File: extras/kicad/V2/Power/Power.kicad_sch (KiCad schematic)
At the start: 73 parts, among them J1 Conn_01x02, J2 Screw_Terminal_01x06, J3 Screw_Terminal_01x06, J4 Screw_Terminal_01x06, J5 Screw_Terminal_01x06, J6 Conn_02x20_Odd_Even, J7 Conn_02x20_Odd_Even, U1 TB6612FNG, U2 TB6612FNG, U3 TPS5430DDAR, U4 TPS5430DDAR

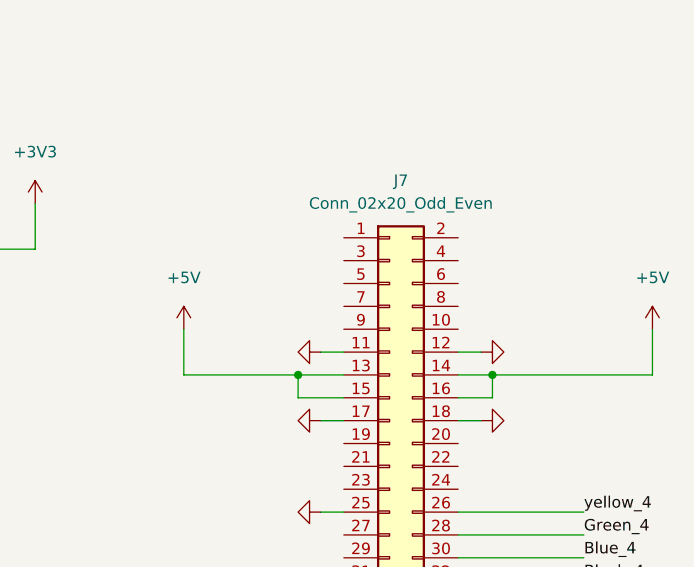
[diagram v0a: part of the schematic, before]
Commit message: g
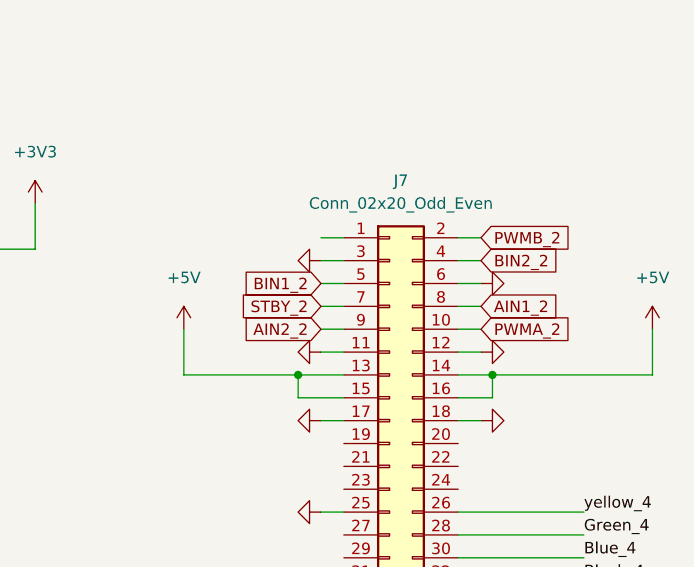
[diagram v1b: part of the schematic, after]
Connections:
- net AIN1_2: now also J7.8 (Pin_8)
- net AIN2_2: now also J7.9 (Pin_9)
- net BIN1_2: now also J7.5 (Pin_5)
- net BIN2_2: now also J7.4 (Pin_4)
- net GND: now also J7.3 (Pin_3), J7.6 (Pin_6)
- net PWMA_2: now also J7.10 (Pin_10)
- net PWMB_2: now also J7.2 (Pin_2)
- net STBY_2: now also J7.7 (Pin_7)
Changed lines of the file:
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@@
     (stroke (width 0) (type default) (color 0 0 0 0))
   )
+  (wire (pts (xy 363.22 119.38) (xy 365.76 119.38))
+    (stroke (width 0) (type default) (color 0 0 0 0))
+  )
+  (wire (pts (xy 363.22 124.46) (xy 365.76 124.46))
+    (stroke (width 0) (type default) (color 0 0 0 0))
+  )
   (wire (pts (xy 34.29 163.83) (xy 38.1 163.83))
     (stroke (width 0) (type default) (color 0 0 0 0))
@@
     (stroke (width 0) (type default) (color 0 0 0 0))
   )
+  (wire (pts (xy 378.46 124.46) (xy 381 124.46))
+    (stroke (width 0) (type default) (color 0 0 0 0))
+  )
   (wire (pts (xy 173.99 163.83) (xy 173.99 166.37))
     (stroke (width 0) (type default) (color 0 0 0 0))
@@
     (stroke (width 0) (type default) (color 0 0 0 0))
   )
+  (wire (pts (xy 378.46 129.54) (xy 381 129.54))
+    (stroke (width 0) (type default) (color 0 0 0 0))
+  )
   (wire (pts (xy 44.45 212.09) (xy 86.36 212.09))
     (stroke (width 0) (type default) (color 0 0 0 0))
@@
     (stroke (width 0) (type default) (color 0 0 0 0))
   )
+  (wire (pts (xy 363.22 127) (xy 365.76 127))
+    (stroke (width 0) (type default) (color 0 0 0 0))
+  )
   (wire (pts (xy 133.35 175.26) (xy 133.35 176.53))
     (stroke (width 0) (type default) (color 0 0 0 0))
@@
     (stroke (width 0) (type default) (color 0 0 0 0))
   )
+  (wire (pts (xy 363.22 121.92) (xy 365.76 121.92))
+    (stroke (width 0) (type default) (color 0 0 0 0))
+  )
   (wire (pts (xy 43.18 46.99) (xy 46.99 46.99))
     (stroke (width 0) (type default) (color 0 0 0 0))
@@
     (stroke (width 0) (type default) (color 0 0 0 0))
   )
+  (wire (pts (xy 378.46 119.38) (xy 381 119.38))
+    (stroke (width 0) (type default) (color 0 0 0 0))
+  )
+  (wire (pts (xy 378.46 127) (xy 381 127))
+    (stroke (width 0) (type default) (color 0 0 0 0))
+  )
   (wire (pts (xy 303.53 123.19) (xy 303.53 120.65))
     (stroke (width 0) (type default) (color 0 0 0 0))
@@
     (stroke (width 0) (type default) (color 0 0 0 0))
   )
+  (wire (pts (xy 363.22 129.54) (xy 365.76 129.54))
+    (stroke (width 0) (type default) (color 0 0 0 0))
+  )
   (wire (pts (xy 361.95 74.93) (xy 370.84 74.93))
     (stroke (width 0) (type default) (color 0 0 0 0))
@@
     (stroke (width 0) (type default) (color 0 0 0 0))
   )
+  (wire (pts (xy 378.46 121.92) (xy 381 121.92))
+    (stroke (width 0) (type default) (color 0 0 0 0))
+  )
   (wire (pts (xy 127 83.82) (xy 118.11 83.82))
     (stroke (width 0) (type default) (color 0 0 0 0))
@@
     )
   )
+  (global_label "PWMA_2" (shape input) (at 381 129.54 0) (fields_autoplaced)
+    (effects (font (size 1.27 1.27)) (justify left))
+    (property "Intersheet References" "${INTERSHEET_REFS}" (id 0) (at 390.8517 129.4606 0)
+      (effects (font (size 1.27 1.27)) (justify left) hide)
+    )
+  )
   (global_label "AIN2_2" (shape input) (at 171.45 93.98 180) (fields_autoplaced)
     (effects (font (size 1.27 1.27)) (justify right))
@@
     )
   )
+  (global_label "STBY_2" (shape input) (at 363.22 127 180) (fields_autoplaced)
+    (effects (font (size 1.27 1.27)) (justify right))
+    (property "Intersheet References" "${INTERSHEET_REFS}" (id 0) (at 354.094 126.9206 0)
+      (effects (font (size 1.27 1.27)) (justify right) hide)
+    )
+  )
   (global_label "BIN1_1" (shape input) (at 80.01 96.52 180) (fields_autoplaced)
     (effects (font (size 1.27 1.27)) (justify right))
@@
     )
   )
+  (global_label "AIN1_2" (shape input) (at 381 127 0) (fields_autoplaced)
+    (effects (font (size 1.27 1.27)) (justify left))
+    (property "Intersheet References" "${INTERSHEET_REFS}" (id 0) (at 389.8236 127.0794 0)
+      (effects (font (size 1.27 1.27)) (justify left) hide)
+    )
+  )
+  (global_label "BIN1_2" (shape input) (at 363.22 124.46 180) (fields_autoplaced)
+    (effects (font (size 1.27 1.27)) (justify right))
+    (property "Intersheet References" "${INTERSHEET_REFS}" (id 0) (at 354.215 124.3806 0)
+      (effects (font (size 1.27 1.27)) (justify right) hide)
+    )
+  )
   (global_label "STBY_2" (shape input) (at 172.72 78.74 180) (fields_autoplaced)
     (effects (font (size 1.27 1.27)) (justify right))
@@
     )
   )
+  (global_label "PWMB_2" (shape input) (at 381 119.38 0) (fields_autoplaced)
+    (effects (font (size 1.27 1.27)) (justify left))
+    (property "Intersheet References" "${INTERSHEET_REFS}" (id 0) (at 391.0331 119.4594 0)
+      (effects (font (size 1.27 1.27)) (justify left) hide)
+    )
+  )
   (global_label "BIN1_2" (shape input) (at 171.45 96.52 180) (fields_autoplaced)
     (effects (font (size 1.27 1.27)) (justify right))
@@
     )
   )
+  (global_label "BIN2_2" (shape input) (at 381 121.92 0) (fields_autoplaced)
+    (effects (font (size 1.27 1.27)) (justify left))
+    (property "Intersheet References" "${INTERSHEET_REFS}" (id 0) (at 390.005 121.9994 0)
+      (effects (font (size 1.27 1.27)) (justify left) hide)
+    )
+  )
   (global_label "AIN1_1" (shape input) (at 80.01 91.44 180) (fields_autoplaced)
     (effects (font (size 1.27 1.27)) (justify right))
@@
     )
   )
+  (global_label "AIN2_2" (shape input) (at 363.22 129.54 180) (fields_autoplaced)
+    (effects (font (size 1.27 1.27)) (justify right))
+    (property "Intersheet References" "${INTERSHEET_REFS}" (id 0) (at 354.3964 129.6194 0)
+      (effects (font (size 1.27 1.27)) (justify right) hide)
+    )
+  )
   (symbol (lib_id "power:GND") (at 110.49 116.84 0) (unit 1)
     (in_bom yes) (on_board yes) (fields_autoplaced)
@@
     (pin "1")
   )
+  (symbol (lib_id "power:GND") (at 381 124.46 90) (unit 1)
+    (in_bom yes) (on_board yes) (fields_autoplaced)
+    (property "Reference" "#PWR0129" (id 0) (at 387.35 124.46 0)
+      (effects (font (size 1.27 1.27)) hide)
+    )
+    (property "Value" "GND" (id 1) (at 385.445 124.46 0)
+      (effects (font (size 1.27 1.27)) hide)
+    )
+    (property "Footprint" "" (id 2) (at 381 124.46 0)
+      (effects (font (size 1.27 1.27)) hide)
+    )
+    (property "Datasheet" "" (id 3) (at 381 124.46 0)
+      (effects (font (size 1.27 1.27)) hide)
+    )
+    (pin "1")
+  )
   (symbol (lib_id "Device:C_Small") (at 220.98 66.04 0) (unit 1)
     (in_bom yes) (on_board yes) (fields_autoplaced)
@@
     (pin "1")
   )
+  (symbol (lib_id "power:GND") (at 363.22 121.92 270) (unit 1)
+    (in_bom yes) (on_board yes) (fields_autoplaced)
+    (property "Reference" "#PWR0130" (id 0) (at 356.87 121.92 0)
+      (effects (font (size 1.27 1.27)) hide)
+    )
+    (property "Value" "GND" (id 1) (at 358.775 121.92 0)
+      (effects (font (size 1.27 1.27)) hide)
+    )
+    (property "Footprint" "" (id 2) (at 363.22 121.92 0)
+      (effects (font (size 1.27 1.27)) hide)
+    )
+    (property "Datasheet" "" (id 3) (at 363.22 121.92 0)
+      (effects (font (size 1.27 1.27)) hide)
+    )
+    (pin "1")
+  )
   (symbol (lib_id "Driver_Motor:TB6612FNG") (at 102.87 88.9 0) (unit 1)
     (in_bom yes) (on_board yes) (fields_autoplaced)
@@
       (reference "#PWR0128") (unit 1) (value "GND") (footprint "")
     )
+    (path "/2c3c323e-076a-48be-8528-4ec91429e42a"
+      (reference "#PWR0129") (unit 1) (value "GND") (footprint "")
+    )
+    (path "/6008c2a9-ed79-4afa-b1aa-7816935a796a"
+      (reference "#PWR0130") (unit 1) (value "GND") (footprint "")
+    )
     (path "/3e61f6a5-00f4-42da-a66c-ad8e9078406a"

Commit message: n
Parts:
- removed R1: R_Small, symbol Device:R_Small
- added TP3, TP4, TP5, TP6: TestPoint, TestPoint:TestPoint_Pad_D1.0mm, symbol Connector:TestPoint
- added U5: INA219AxD, Package_SO:SOIC-8_3.9x4.9mm_P1.27mm, symbol Analog_ADC:INA219AxD
- C1: value 1n5 -> 100n; footprint Capacitor_SMD:C_0603_1608Metric_Pad1.08x0.95mm_HandSolder -> Capacitor_SMD:C_0603_1608Metric; LCSC (none) -> C14663
- J6: value Conn_02x20_Odd_Even -> left
- J7: value Conn_02x20_Odd_Even -> right
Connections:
- net +12V: now also C1.1, TP4.1, U5.7 (IN-)
- net +5V: now also C2.2, U5.5 (VS)
- net AIN1_1: now also J6.39 (Pin_39)
- net AIN2_1: now also J6.37 (Pin_37)
- net AO1_1: now also J3.1 (Pin_1); no longer J3.6 (Pin_6)
- net AO1_2: now also J4.2 (Pin_2); no longer J4.5 (Pin_5)
- net AO2_1: now also J3.2 (Pin_2); no longer J3.5 (Pin_5)
- net AO2_2: now also J4.1 (Pin_1); no longer J4.6 (Pin_6)
- net BIN1_1: now also J6.34 (Pin_34)
- net BIN2_1: now also J6.36 (Pin_36)
- net Black_1: now also J6.33 (Pin_33); no longer J6.39 (Pin_39)
- net Black_2: now also J3.6 (Pin_6), J6.21 (Pin_21); no longer J3.1 (Pin_1), J6.31 (Pin_31)
- net Black_3: now also J4.6 (Pin_6); no longer J4.1 (Pin_1)
- net Blue_1: now also J6.31 (Pin_31); no longer J6.37 (Pin_37)
- net Blue_2: now also J3.5 (Pin_5), J6.19 (Pin_19); no longer J3.2 (Pin_2), J6.29 (Pin_29)
- net Blue_3: now also J4.5 (Pin_5); no longer J4.2 (Pin_2)
- net GND: now also C2.1, J6.16 (Pin_16), J6.20 (Pin_20), J6.25 (Pin_25), TP5.1, TP6.1, U5.1 (A1), U5.2 (A0), U5.6 (GND)
- net Green_1: now also J6.29 (Pin_29); no longer J6.35 (Pin_35)
- net Green_2: now also J3.4 (Pin_4), J6.17 (Pin_17); no longer J3.3 (Pin_3), J6.27 (Pin_27)
- net Green_3: now also J4.4 (Pin_4); no longer J4.3 (Pin_3)
- net PWMA_1: now also J6.35 (Pin_35)
- net PWMB_1: now also J6.40 (Pin_40)
- net STBY_1: now also J6.30 (Pin_30)
- net yellow_1: now also J6.27 (Pin_27); no longer J6.33 (Pin_33)
- net yellow_2: now also J3.3 (Pin_3), J6.15 (Pin_15); no longer J3.4 (Pin_4), J6.25 (Pin_25)
- net yellow_3: now also J4.3 (Pin_3); no longer J4.4 (Pin_4)
- net at J1.2 (Pin_2), R12.1, R13.1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: now also C1.2, TP3.1, U5.8 (IN+)
- net SCL: now reaches J6.1 (Pin_1)
- net SCL: now also U5.4 (SCL)
- net SDA: now reaches J6.2 (Pin_2)
- net SDA: now also U5.3 (SDA)
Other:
- moved on the sheet: C10, C11, C3, C4, C5, C6, C7, C8, C9, H1, H10, H11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
